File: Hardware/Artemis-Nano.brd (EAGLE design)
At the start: 43.2 x 20.3 mm, 129 parts, among them J10 USB-C, J11 CORTEX_DEBUG, U2 MCP73831, U3 3.3V, U4 ARTEMIS_MODULESMD, U6 CH340E_MSOP10, Y2 32.768kHz

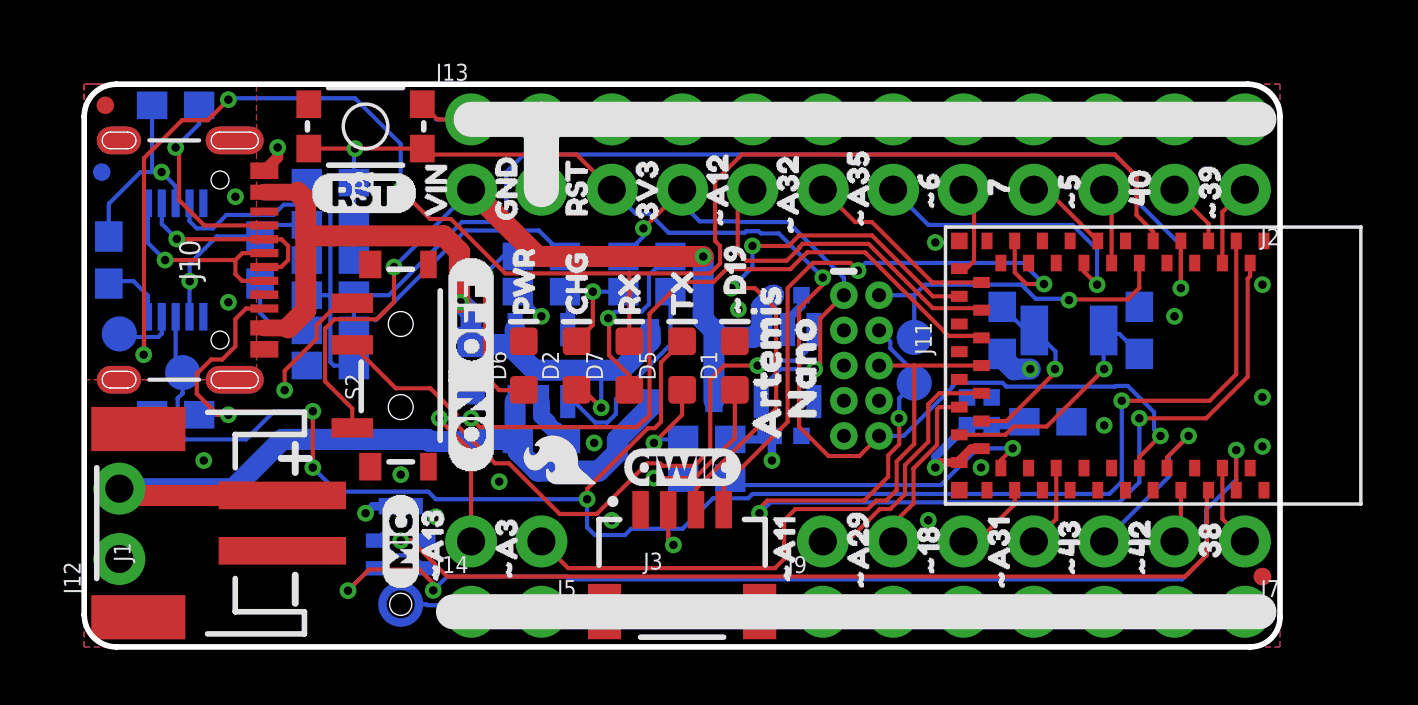
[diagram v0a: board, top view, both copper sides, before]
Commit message: Rename to Nano. Add ignore. Add panel.
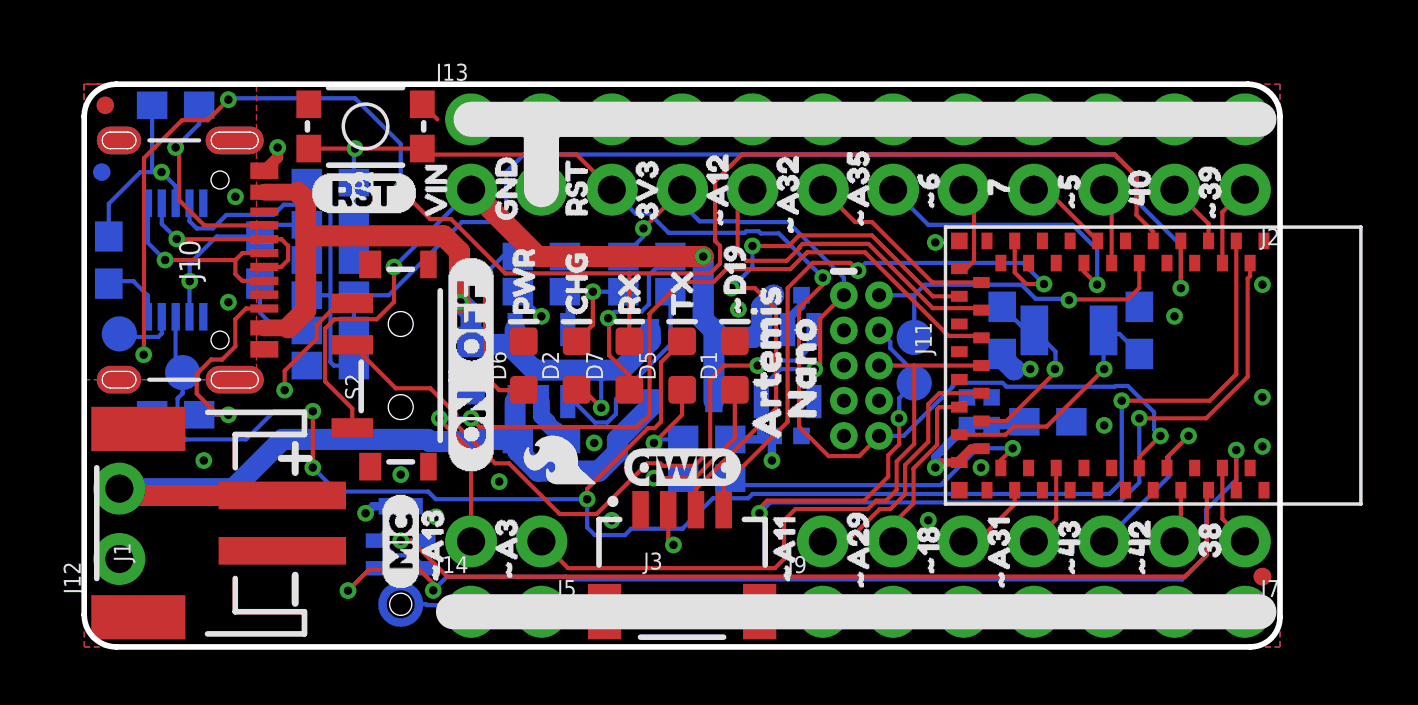
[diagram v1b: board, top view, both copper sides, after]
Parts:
- removed LOGO2: OSHW-LOGOS, SparkFun-Aesthetics:OSHW-LOGO-S
- removed LOGO3: SFE_LOGO_NAME_FLAME.1_INCH, SparkFun-Aesthetics:SFE_LOGO_NAME_FLAME_.1
- added U$25: (no value), SparkFun-Aesthetics:PRODUCTION_INSTRUCTIONS
- moved FRAME2 55.3 mm to (0.00, 0.00)
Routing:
- net 3.3V: track 50.7 -> 46.9 mm
- net GND: track 31.5 -> 28.7 mm
- added copper zone on layer 15, net 3.3V
- added copper zone on layer 2, net GND
- removed copper zone on layer 2, net 3.3V
- removed copper zone on layer 15, net GND
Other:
- board text added: "0.8mm Thickness"
- board text added: "Four-layer board"
